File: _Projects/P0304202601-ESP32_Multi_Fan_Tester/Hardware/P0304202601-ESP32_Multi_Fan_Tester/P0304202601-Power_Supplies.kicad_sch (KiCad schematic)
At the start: 3 parts, among them CN3 KJ694108301002, IC1 PMAP63205WU-7

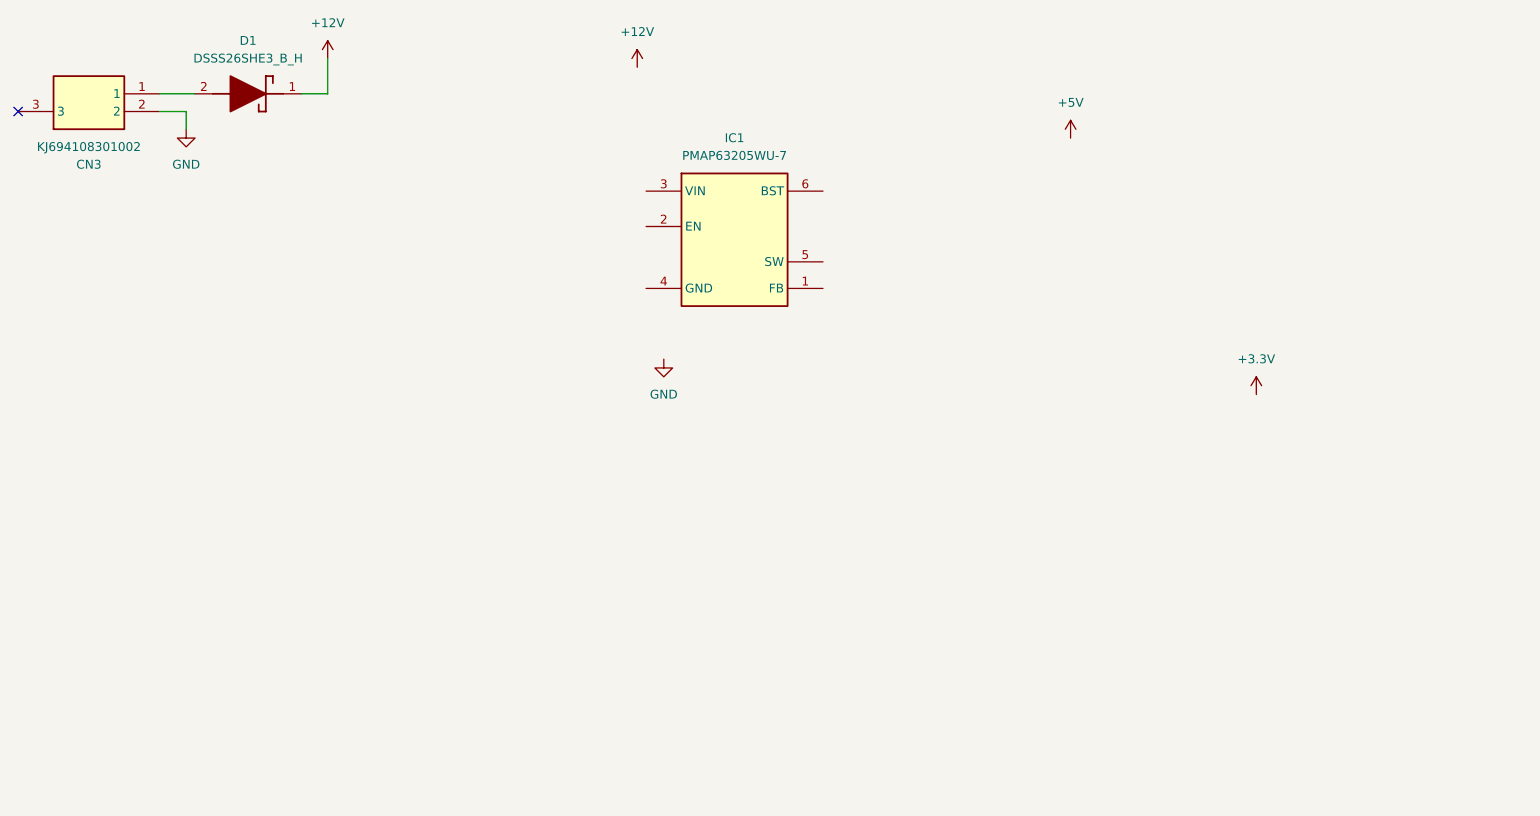
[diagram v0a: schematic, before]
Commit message: Added new content from recent stream.
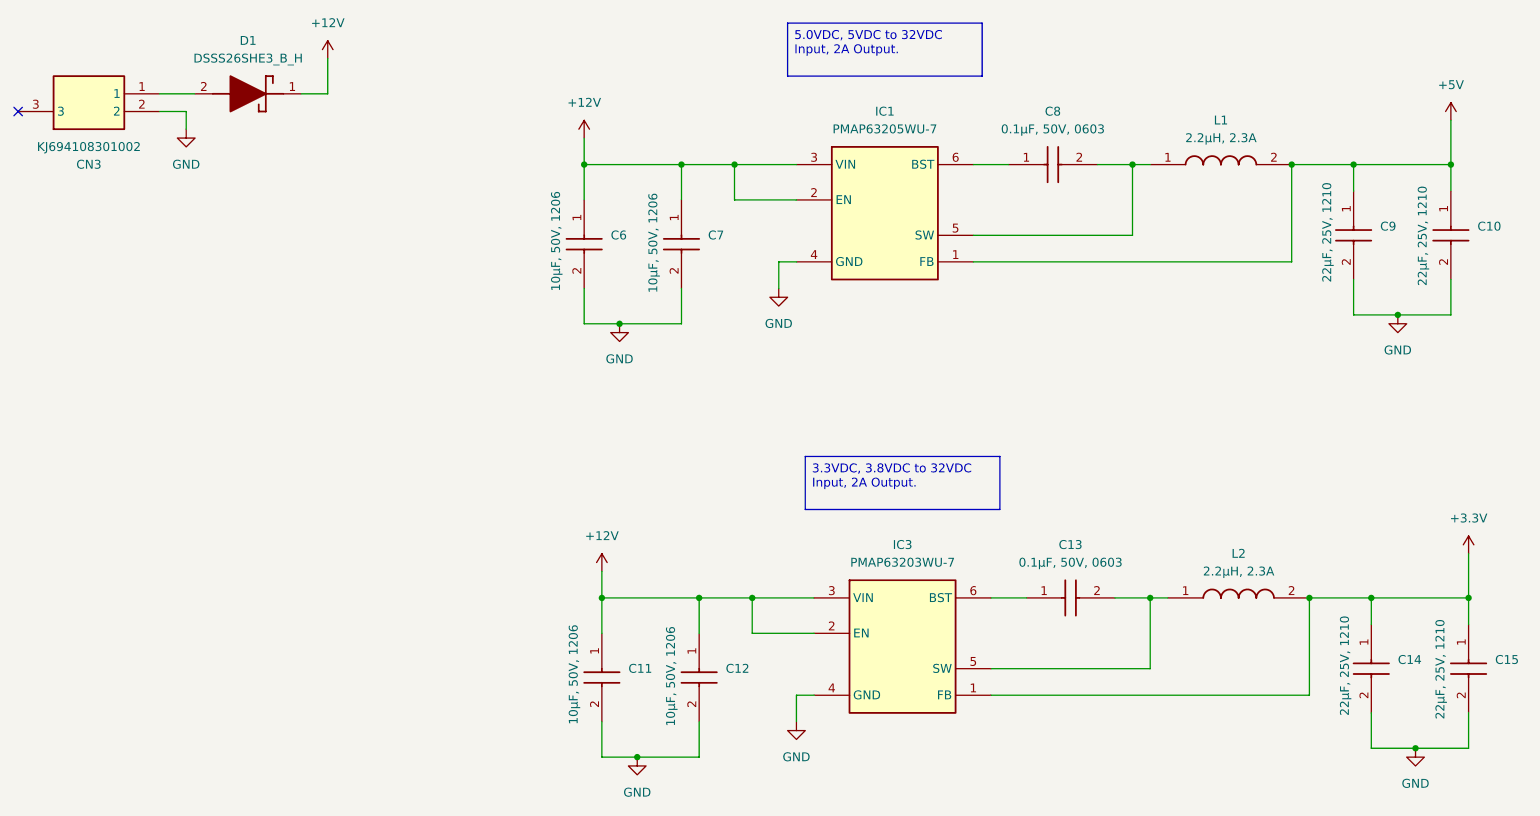
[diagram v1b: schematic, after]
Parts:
- added C10, C14, C15, C9: CC1210226025AAAX7R, COMPONENTS:CAP-1210, symbol COMPONENTS:CC1210226025AAAX7R
- added C11, C12, C6, C7: CC1206106050AAAX7R, COMPONENTS:CAP-1206, symbol COMPONENTS:CC1206106050AAAX7R
- added C13, C8: CC0603104050AAAX7R, COMPONENTS:CAP-0603, symbol COMPONENTS:CC0603104050AAAX7R
- added IC3: PMAP63203WU-7, COMPONENTS:TSOT-26-6, symbol COMPONENTS:PMAP63203WU-7
- added L1, L2: LSRP2512-2R2M, COMPONENTS:IND-1005, symbol COMPONENTS:LSRP2512-2R2M
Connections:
- net +12V: now also IC1.2 (EN), IC1.3 (VIN), C11.1, C12.1, C6.1, C7.1, IC3.2 (EN), IC3.3 (VIN)
- net +3.3V: now also C14.1, C15.1, IC3.1 (FB), L2.2
- net +5V: now also IC1.1 (FB), C10.1, C9.1, L1.2
- net GND: now also IC1.4 (GND), C10.2, C11.2, C12.2, C14.2, C15.2, C6.2, C7.2, C9.2, IC3.4 (GND)
- net at IC1.5 (SW): now also C8.2, L1.1
- net at IC1.6 (BST): now also C8.1
- new net: C13.2, IC3.5 (SW), L2.1
- new net: C13.1, IC3.6 (BST)
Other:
- moved on the sheet: IC1
